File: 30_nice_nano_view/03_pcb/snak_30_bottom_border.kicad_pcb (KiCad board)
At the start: 2 copper layers, 114 x 99 mm, 118 parts

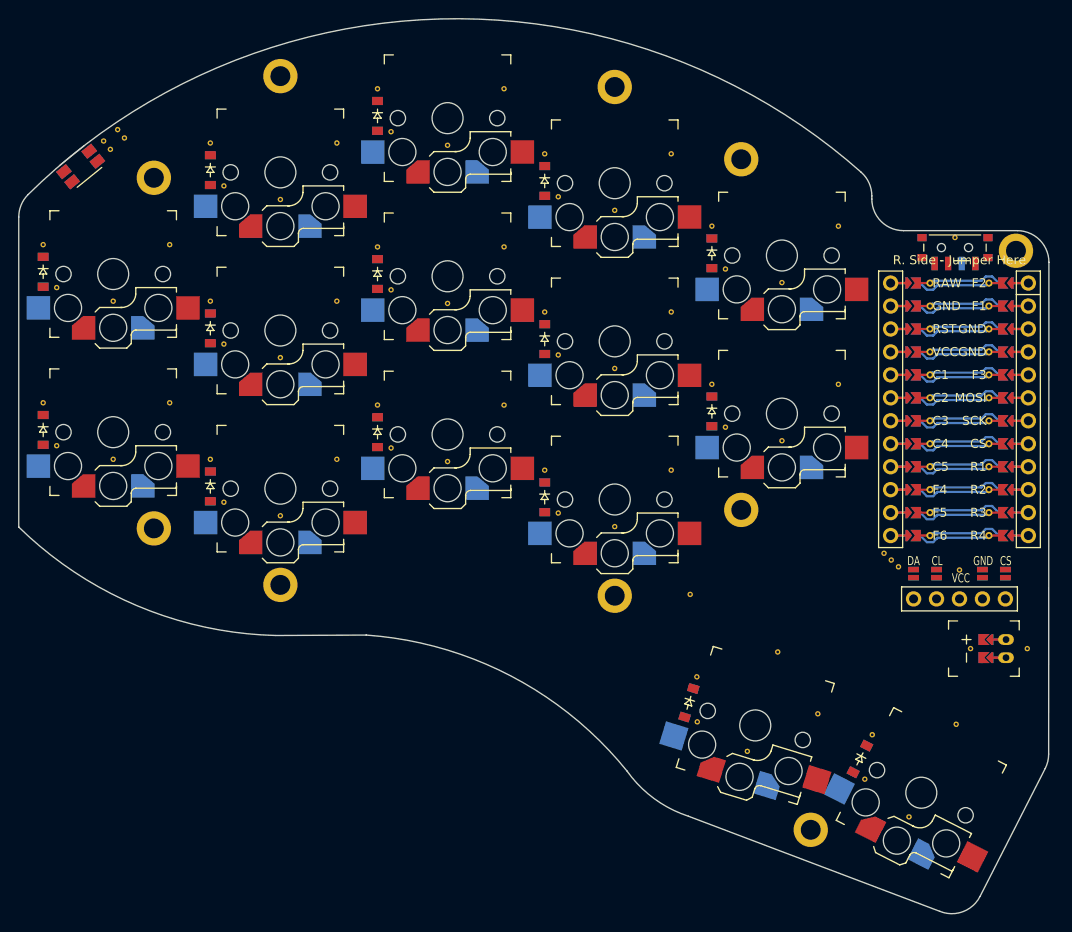
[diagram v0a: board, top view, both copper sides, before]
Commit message: update 30 key nicenano board
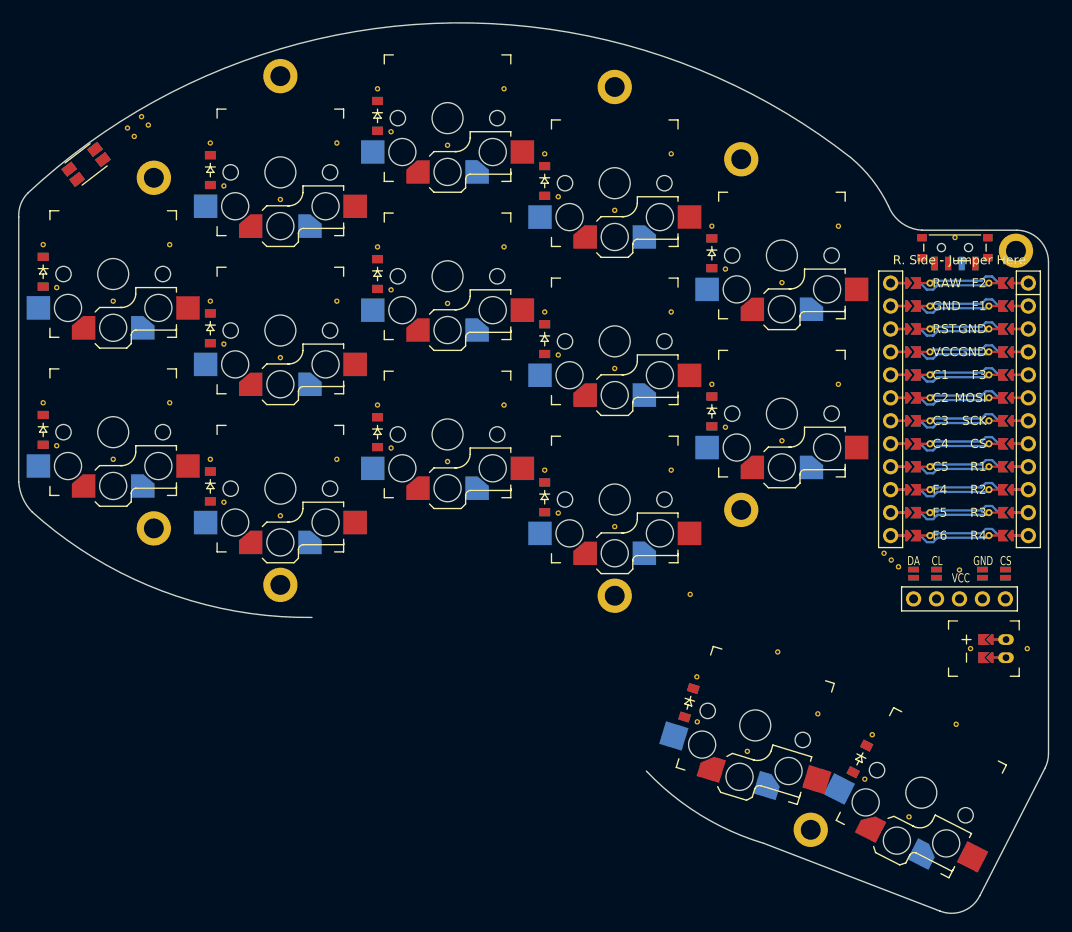
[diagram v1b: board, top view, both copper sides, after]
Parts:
- moved REF** 3.00 mm to (101.6, 48.8)
- moved REF** 3.00 mm to (102.3, 49.8)
- moved REF** 3.00 mm to (103.1, 47.6)
- moved REF** 3.00 mm to (103.9, 48.5)
- moved SW2 0.64 mm to (97.0, 52.9), turned to 127.5 degrees
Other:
- board size 114 x 99 mm -> 114 x 98.5 mm
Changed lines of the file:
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@@
   )
   (footprint "VIA-0.6mm" (layer "F.Cu")
-    (at 100.494144 49.019006 129)
+    (at 103.137109 47.589196 129)
     (attr through_hole)
     (fp_text reference "REF**" (at 0 1.4) (layer "F.SilkS") hide
@@
   )
   (footprint "VIA-0.6mm" (layer "F.Cu")
-    (at 101.243035 49.94381 129)
+    (at 103.886 48.514 129)
     (attr through_hole)
     (fp_text reference "REF**" (at 0 1.4) (layer "F.SilkS") hide
@@
   )
   (footprint "VIA-0.6mm" (layer "F.Cu")
-    (at 98.939852 50.277647 129)
+    (at 101.582817 48.847837 129)
     (attr through_hole)
     (fp_text reference "REF**" (at 0 1.4) (layer "F.SilkS") hide
@@
   )
   (footprint "sw_reset_side" (layer "F.Cu")
-    (at 96.4 53.1 129)
+    (at 97 52.87 127.5)
     (attr smd)
-    (fp_text reference "SW2" (at 0 3.5 129) (layer "F.SilkS") hide
+    (fp_text reference "SW2" (at 0 3.5 127.5) (layer "F.SilkS") hide
         (effects (font (size 1 1) (thickness 0.15)))
     )
-    (fp_text value "" (at 0 0 129) (layer "F.SilkS")
+    (fp_text value "" (at 0 0 127.5) (layer "F.SilkS")
         (effects (font (size 1.27 1.27) (thickness 0.15)))
     )
-    (fp_text user "SW2" (at 0 3.5 129) (layer "B.SilkS") hide
+    (fp_text user "SW2" (at 0 3.5 127.5) (layer "B.SilkS") hide
         (effects (font (size 1 1) (thickness 0.15)) (justify mirror))
     )
@@
     (fp_line (start 2.1 0.85) (end 2.1 -0.85)
       (stroke (width 0.1) (type solid)) (layer "F.Fab"))
-    (pad "1" smd rect (at -0.72 -1.8 219) (size 1.4 1.05) (layers "F.Cu" "F.Paste" "F.Mask")
+    (pad "1" smd rect (at -0.72 -1.8 217.5) (size 1.4 1.05) (layers "F.Cu" "F.Paste" "F.Mask")
       (net 26 "GND"))
-    (pad "1" smd rect (at -0.72 -1.8 39) (size 1.4 1.05) (layers "B.Cu" "B.Paste" "B.Mask")
+    (pad "1" smd rect (at -0.72 -1.8 37.5) (size 1.4 1.05) (layers "B.Cu" "B.Paste" "B.Mask")
       (net 26 "GND"))
-    (pad "1" smd rect (at -0.72 1.8 219) (size 1.4 1.05) (layers "F.Cu" "F.Paste" "F.Mask")
+    (pad "1" smd rect (at -0.72 1.8 217.5) (size 1.4 1.05) (layers "F.Cu" "F.Paste" "F.Mask")
       (net 26 "GND"))
-    (pad "1" smd rect (at -0.72 1.8 39) (size 1.4 1.05) (layers "B.Cu" "B.Paste" "B.Mask")
+    (pad "1" smd rect (at -0.72 1.8 37.5) (size 1.4 1.05) (layers "B.Cu" "B.Paste" "B.Mask")
       (net 26 "GND"))
-    (pad "2" smd rect (at 0.72 -1.8 219) (size 1.4 1.05) (layers "F.Cu" "F.Paste" "F.Mask")
+    (pad "2" smd rect (at 0.72 -1.8 217.5) (size 1.4 1.05) (layers "F.Cu" "F.Paste" "F.Mask")
       (net 27 "RST"))
-    (pad "2" smd rect (at 0.72 -1.8 39) (size 1.4 1.05) (layers "B.Cu" "B.Paste" "B.Mask")
+    (pad "2" smd rect (at 0.72 -1.8 37.5) (size 1.4 1.05) (layers "B.Cu" "B.Paste" "B.Mask")
       (net 27 "RST"))
-    (pad "2" smd rect (at 0.72 1.8 219) (size 1.4 1.05) (layers "F.Cu" "F.Paste" "F.Mask")
+    (pad "2" smd rect (at 0.72 1.8 217.5) (size 1.4 1.05) (layers "F.Cu" "F.Paste" "F.Mask")
       (net 27 "RST"))
-    (pad "2" smd rect (at 0.72 1.8 39) (size 1.4 1.05) (layers "B.Cu" "B.Paste" "B.Mask")
+    (pad "2" smd rect (at 0.72 1.8 37.5) (size 1.4 1.05) (layers "B.Cu" "B.Paste" "B.Mask")
       (net 27 "RST"))
   )
@@
   )
   (footprint "VIA-0.6mm" (layer "F.Cu")
-    (at 99.688743 51.20245 129)
+    (at 102.331708 49.77264 129)
     (attr through_hole)
     (fp_text reference "REF**" (at 0 1.4) (layer "F.SilkS") hide
@@
   (gr_circle (center 118.5 99.4) (end 120 99.4)
     (stroke (width 0.15) (type solid)) (fill none) (layer "Eco2.User"))
-  (gr_line (start 203.13565 119.719514) (end 195.923145 133.874853)
+  (gr_arc (start 172 128) (mid 164.97339 124.855741) (end 159 120)
     (stroke (width 0.15) (type solid)) (layer "Edge.Cuts"))
-  (gr_arc (start 187.45 60.2) (mid 184.975126 59.174874) (end 183.95 56.7)
+  (gr_line (start 203.1 119.7) (end 195.9 133.8)
     (stroke (width 0.15) (type solid)) (layer "Edge.Cuts"))
-  (gr_line (start 89.55 93) (end 89.55 58.692372)
+  (gr_arc (start 189.5 60.15) (mid 187.263797 59.364226) (end 185.8 57.5)
     (stroke (width 0.15) (type solid)) (layer "Edge.Cuts"))
-  (gr_arc (start 163.66 124.999999) (mid 159.844543 123.03625) (end 156.839956 119.972513)
+  (gr_line (start 89.55 88) (end 89.55 58.7)
     (stroke (width 0.15) (type solid)) (layer "Edge.Cuts"))
-  (gr_line (start 187.45 60.2) (end 200.048013 60.2)
+  (gr_line (start 189.5 60.15) (end 200 60.15)
     (stroke (width 0.15) (type solid)) (layer "Edge.Cuts"))
-  (gr_arc (start 89.55 58.692372) (mid 89.820936 57.342133) (end 90.591797 56.200939)
+  (gr_arc (start 89.55 58.7) (mid 89.780852 57.235609) (end 90.6 56)
     (stroke (width 0.15) (type solid)) (layer "Edge.Cuts"))
-  (gr_arc (start 203.517127 118.132533) (mid 203.42019 118.948572) (end 203.13565 119.719514)
+  (gr_arc (start 203.5 118.1) (mid 203.39457 118.923643) (end 203.1 119.7)
     (stroke (width 0.15) (type solid)) (layer "Edge.Cuts"))
-  (gr_line (start 183.95 56.7) (end 183.95 56.354306)
+  (gr_line (start 203.5 63.7) (end 203.5 118.1)
     (stroke (width 0.15) (type solid)) (layer "Edge.Cuts"))
-  (gr_line (start 203.548013 63.701986) (end 203.517127 118.132533)
+  (gr_arc (start 91 91.3) (mid 89.98406 89.777837) (end 89.55 88)
     (stroke (width 0.15) (type solid)) (layer "Edge.Cuts"))
-  (gr_arc (start 195.923145 133.874853) (mid 194.021857 135.567401) (end 191.476715 135.524198)
+  (gr_arc (start 195.9 133.8) (mid 194.031815 135.508815) (end 191.5 135.5)
     (stroke (width 0.15) (type solid)) (layer "Edge.Cuts"))
-  (gr_arc (start 200.048013 60.199999) (mid 202.523589 61.225828) (end 203.548013 63.701986)
+  (gr_arc (start 200 60.15) (mid 202.485523 61.199837) (end 203.5 63.7)
     (stroke (width 0.15) (type solid)) (layer "Edge.Cuts"))
-  (gr_arc (start 118 105) (mid 102.635557 101.701429) (end 89.55 93)
+  (gr_arc (start 181.6 52.1) (mid 183.995505 54.570163) (end 185.8 57.5)
     (stroke (width 0.15) (type solid)) (layer "Edge.Cuts"))
-  (gr_arc (start 182.771484 53.73501) (mid 183.641801 54.918199) (end 183.95 56.354306)
+  (gr_arc (start 90.6 56) (mid 135.380905 37.271116) (end 181.6 52.1)
     (stroke (width 0.15) (type solid)) (layer "Edge.Cuts"))
-  (gr_line (start 128.003322 104.952626) (end 118 105)
+  (gr_line (start 191.5 135.5) (end 172 128)
     (stroke (width 0.15) (type solid)) (layer "Edge.Cuts"))
-  (gr_arc (start 90.591797 56.200939) (mid 136.194931 36.77414) (end 182.771484 53.73501)
-    (stroke (width 0.15) (type solid)) (layer "Edge.Cuts"))
-  (gr_line (start 191.476715 135.524198) (end 163.66 125)
-    (stroke (width 0.15) (type solid)) (layer "Edge.Cuts"))
-  (gr_arc (start 128.003322 104.952626) (mid 143.983857 109.463271) (end 156.839955 119.972514)
+  (gr_arc (start 122 103) (mid 105.398912 100.067413) (end 91 91.3)
     (stroke (width 0.15) (type solid)) (layer "Edge.Cuts"))
+  (gr_arc (start 122 103) (mid 142.325339 107.527204) (end 159 120)
+    (stroke (width 0.15) (type solid)) (layer "F.Fab"))
   (segment (start 198.43 76.16) (end 196.91 76.16) (width 0.25) (layer "F.Cu") (net 1))
   (segment (start 191.11 76.51) (end 191.11 76.5) (width 0.25) (layer "B.Cu") (net 1))
